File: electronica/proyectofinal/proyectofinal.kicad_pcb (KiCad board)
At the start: 2 copper layers, 77 x 67 mm, 16 parts, among them J1 cnn, J2 conector alimentacion esp, J3 dht22, J4 Guva-s12s, J5 convertidor_TTL, J6 MICS-6814, K1 rele 3.3v, K2 rele 5v, U1 LM7833_TO220, U3 LM7805_TO220, U4 ESP32_LORA_V2.0

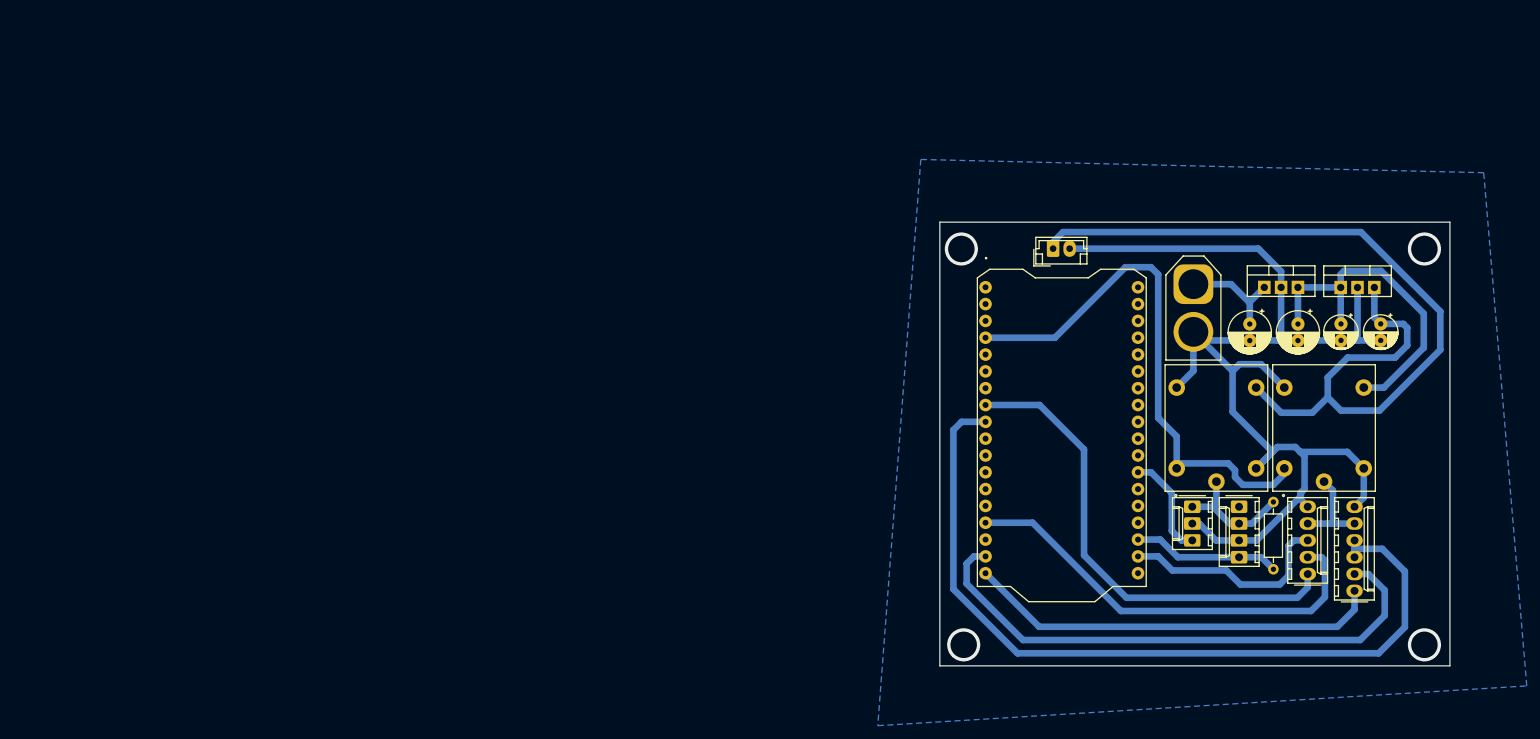
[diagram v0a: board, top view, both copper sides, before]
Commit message: 1
1
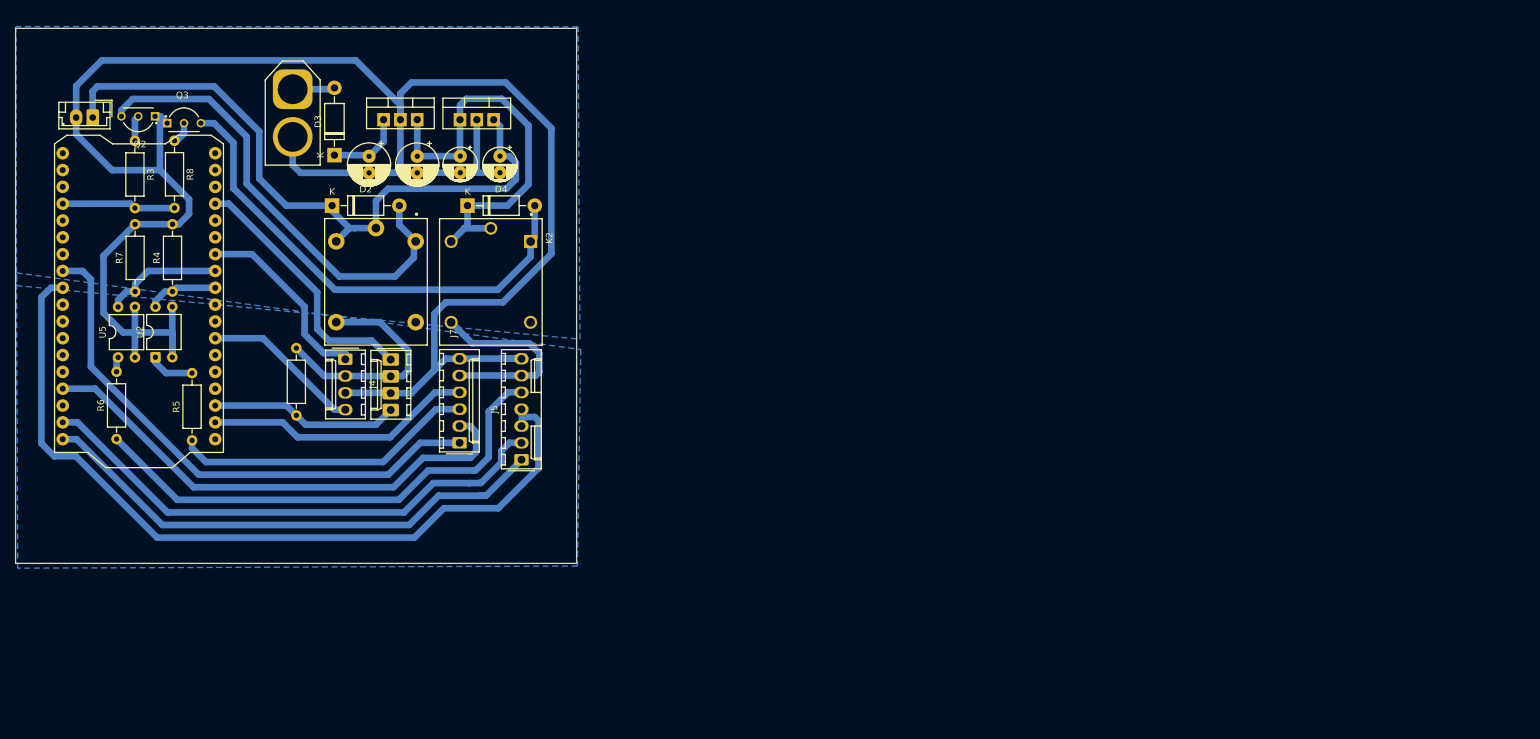
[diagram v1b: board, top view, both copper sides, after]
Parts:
- removed J6: MICS-6814, Connector_Molex:Molex_KK-254_AE-6410-05A_1x05_P2.54mm_Vertical
- added D2: 1N4007, Diode_THT:D_DO-41_SOD81_P10.16mm_Horizontal, F.Cu at (68.6, 46.0)
- added D3: 1N4007, Diode_THT:D_DO-41_SOD81_P10.16mm_Horizontal, F.Cu at (69.0, 38.4)
- added D4: 1N4007, Diode_THT:D_DO-41_SOD81_P10.16mm_Horizontal, F.Cu at (89.1, 46.0)
- added J7: Conn_01x06_Pin, Connector_Molex:Molex_KK-254_AE-6410-06A_1x06_P2.54mm_Vertical, F.Cu at (87.9, 81.9)
- added Q2: 2N2222A, 2N2222A:TO92254P470H750-3, F.Cu at (39.4, 34.9)
- added Q3: 2N2222A, 2N2222A:TO92254P470H750-3, F.Cu at (46.3, 31.3)
- added R3: 330, Resistor_THT:R_Axial_DIN0207_L6.3mm_D2.5mm_P10.16mm_Horizontal, F.Cu at (38.9, 36.3)
- added R4: 30k, Resistor_THT:R_Axial_DIN0207_L6.3mm_D2.5mm_P10.16mm_Horizontal, F.Cu at (44.5, 59.0)
- added R5: 330, Resistor_THT:R_Axial_DIN0207_L6.3mm_D2.5mm_P10.16mm_Horizontal, F.Cu at (47.5, 81.5)
- added R6: 330, Resistor_THT:R_Axial_DIN0207_L6.3mm_D2.5mm_P10.16mm_Horizontal, F.Cu at (36.1, 81.3)
- added R7: 30k, Resistor_THT:R_Axial_DIN0207_L6.3mm_D2.5mm_P10.16mm_Horizontal, F.Cu at (38.9, 59.0)
- added R8: 330, Resistor_THT:R_Axial_DIN0207_L6.3mm_D2.5mm_P10.16mm_Horizontal, F.Cu at (44.9, 36.2)
- added U2: PC817, Package_DIP:DIP-4_W7.62mm, F.Cu at (42.0, 69.0)
- added U5: PC817, Package_DIP:DIP-4_W7.62mm, F.Cu at (36.3, 69.0)
- J4: footprint Connector_Molex:Molex_KK-254_AE-6410-03A_1x03_P2.54mm_Vertical -> Connector_Molex:Molex_KK-254_AE-6410-04A_1x04_P2.54mm_Vertical
- J5: footprint Connector_Molex:Molex_KK-254_AE-6410-06A_1x06_P2.54mm_Vertical -> Connector_Molex:Molex_KK-254_AE-6410-07A_1x07_P2.54mm_Vertical
- K1: value rele 3.3v -> SRD-03VDC-SL-C
- K2: value rele 5v -> SRD-05VDC-SL-C
- moved R1 149.4 mm to (63.2, 77.7)
- moved J2 146.4 mm to (32.5, 32.8), turned to 180 degrees
- moved U4 140.8 mm to (39.5, 60.5)
- moved J1 139.2 mm to (62.7, 28.5)
- moved C1 135.4 mm to (81.5, 38.6)
- moved C2 135.4 mm to (94.0, 38.6)
- moved C3 135.4 mm to (74.2, 38.6)
- moved C4 135.4 mm to (88.0, 38.6)
- moved U1 135.4 mm to (88.0, 33.1)
- moved U3 135.4 mm to (76.4, 33.1)
- moved J3 130.0 mm to (77.5, 69.3)
- moved J4 129.8 mm to (70.7, 69.2)
- moved K1 128.8 mm to (75.3, 57.5), turned to -90 degrees
- moved K2 127.7 mm to (92.6, 57.6), turned to -90 degrees
- moved J5 127.3 mm to (97.2, 84.4)
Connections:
- C3 pad 1: Net-(J1-Pin_1) -> Net-(D3-K)
- J1 pad 1: Net-(J1-Pin_1) -> Net-(D3-A)
- J3 pad 1: unconnected-(J3-Pin_1-Pad1) -> pin dht
- J4 pad 1: +3.3V sensores -> pin Guva-s12s
- J4 pad 2: GND -> +3.3V sensores
- J4 pad 3: SIG_Guva-s12s -> GND
- J5 pad 5: +5V sensores -> bool ttl
- J5 pad 6: GND -> +5V sensores
- K1 pad A1: vext -> Net-(D2-A)
- K1 pad A2: GND -> +3.3V
- K1 pad COM: +3.3V sensores -> +3.3V
- K1 pad NC: GND -> unconnected-(K1-PadNC)
- K1 pad NO: +3.3V -> +3.3V sensores
- K2 pad A1: vext -> Net-(D4-A)
- K2 pad A2: GND -> +5V
- K2 pad COM: +5V sensores -> +5V
- K2 pad NC: GND -> unconnected-(K2-PadNC)
- K2 pad NO: +5V -> +5V sensores
- U3 pad 1: Net-(J1-Pin_1) -> Net-(D3-K)
- U4 pad J3_4: unconnected-(U4-ADC1_0/GPI36/36-PadJ3_4) -> pin dht
- U4 pad J3_7: unconnected-(U4-ADC1_3/GPI39/39-PadJ3_7) -> pin Guva-s12s
- U4 pad J3_8: unconnected-(U4-LORA_DIO2/ADC1_6/GPI34/34-PadJ3_8) -> pin ttl
- U4 pad J3_9: unconnected-(U4-LORA_DIO1/ADC1_7/GPI35/35-PadJ3_9) -> pinmics
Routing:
- net GND: track 182.6 -> 317.2 mm
- net bool ttl: track 0.00 -> 75.8 mm
- net Net-(D4-A): track 0.00 -> 74.3 mm
- net Net-(D2-A): track 0.00 -> 71.2 mm
- net vext: track 81.4 -> 17.2 mm
- net bool mics: track 0.00 -> 45.8 mm
- net pin dht: track 0.00 -> 39.5 mm
- net +3.3V: track 135.6 -> 101.2 mm
- net pin Guva-s12s: track 0.00 -> 29.2 mm
- net pin ttl: track 0.00 -> 18.2 mm
- net +5V sensores: track 14.0 -> 30.4 mm
- net Net-(J1-Pin_1): track 16.1 -> 0.00 mm
- net +3.3V sensores: track 18.7 -> 34.7 mm
- net RO_TTL: track 63.0 -> 78.9 mm
- net Net-(D3-K): track 0.00 -> 11.7 mm
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- added copper zone on B.Cu, net DE/RE_TTL
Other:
- board size 77 x 67 mm -> 84.7 x 80.8 mm

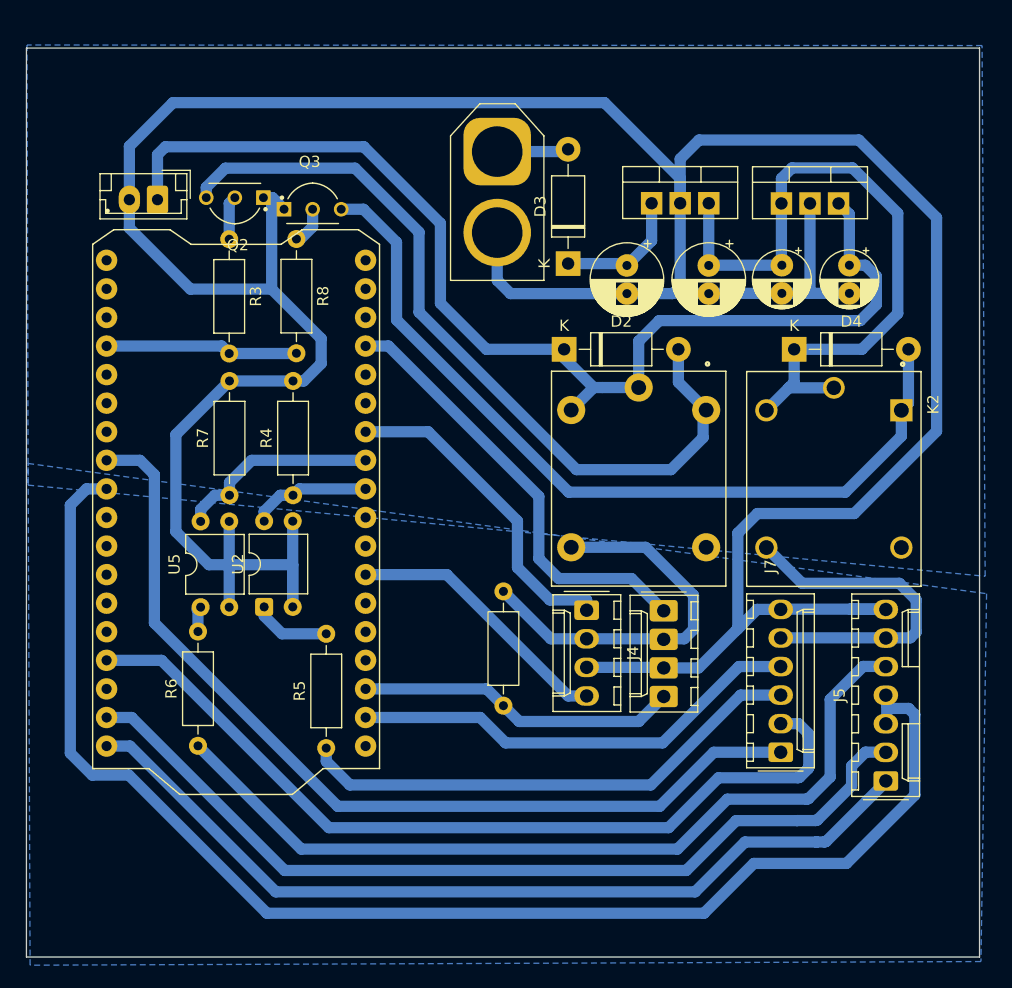
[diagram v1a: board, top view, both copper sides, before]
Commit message: 1
1
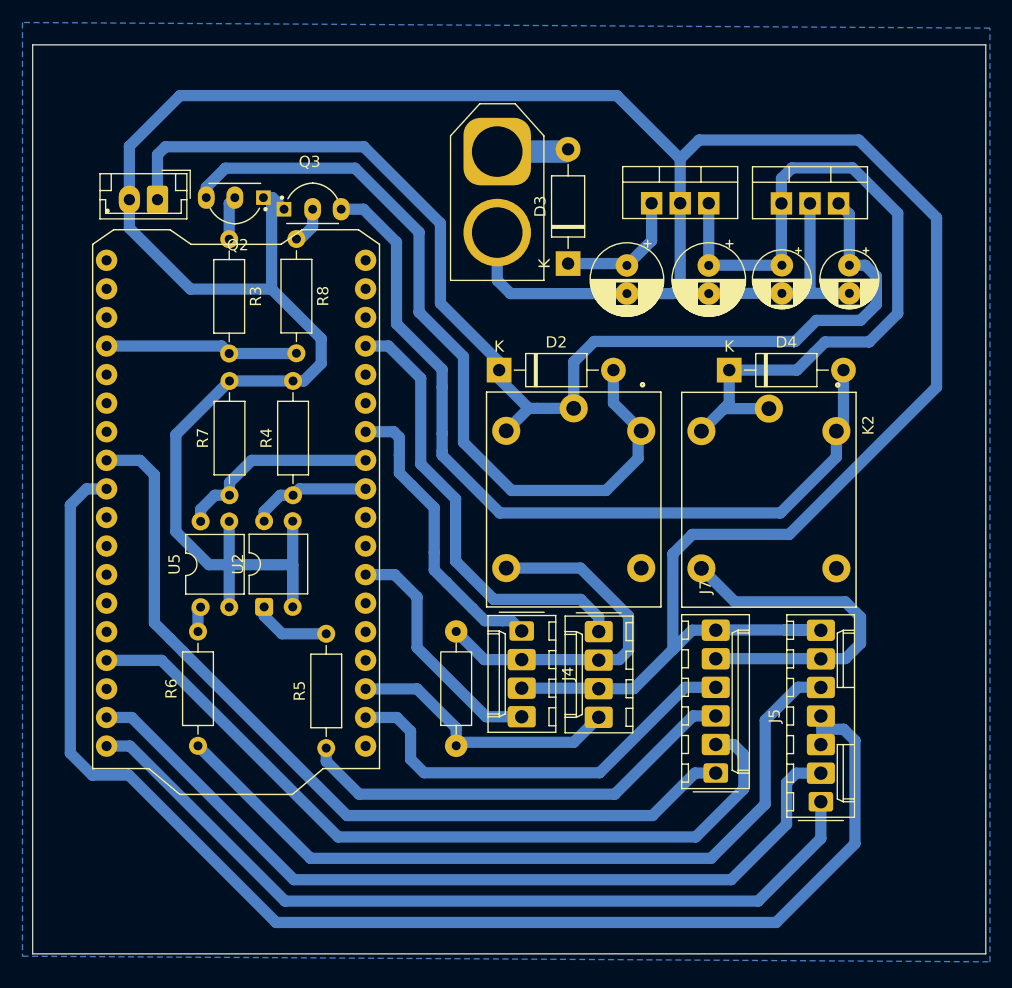
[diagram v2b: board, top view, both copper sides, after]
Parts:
- moved D4 6.06 mm to (83.3, 47.9)
- moved K1 6.06 mm to (69.5, 59.4)
- moved J3 6.06 mm to (71.7, 71.1)
- moved J4 6.06 mm to (64.9, 71.1)
- moved J5 6.06 mm to (91.5, 86.3)
- moved J7 6.06 mm to (82.1, 83.7)
- moved K2 6.06 mm to (86.8, 59.4)
- moved D2 6.06 mm to (62.9, 47.9)
- moved R1 5.51 mm to (59.1, 81.3)
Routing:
- net +5V: track 62.1 -> 68.6 mm
- net bool mics: track 45.8 -> 39.9 mm
- net SIG_NH3_MICS-6814: track 76.7 -> 70.8 mm
- net SIG_Co_MICS-6814: track 82.4 -> 76.5 mm
- net bool ttl: track 75.8 -> 70.3 mm
- net DI_TTL: track 80.4 -> 75.6 mm
- net RO_TTL: track 78.9 -> 74.8 mm
- net SIG_DHT22: track 28.6 -> 24.8 mm
- net DE/RE_TTL: track 123.7 -> 120.0 mm
- net SIG_N02_MICS-6814: track 40.6 -> 37.8 mm
- net pin Guva-s12s: track 29.2 -> 26.3 mm
- net SIG_Guva-s12s: track 24.1 -> 21.7 mm
- net +3.3V sensores: track 34.7 -> 32.4 mm
- net +3.3V: track 101.2 -> 103.1 mm
- net GND: track 317.2 -> 318.7 mm
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- removed copper zone on B.Cu, net DE/RE_TTL
